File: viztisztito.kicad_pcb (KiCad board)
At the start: 2 copper layers, 110 x 102 mm, 77 parts, among them P1 BOARD_CONN, Q1 BC850, U1 VTX-214-010-205, U2 LTV-847, U3 ACS722, U4 MCP3004, U5 TC77

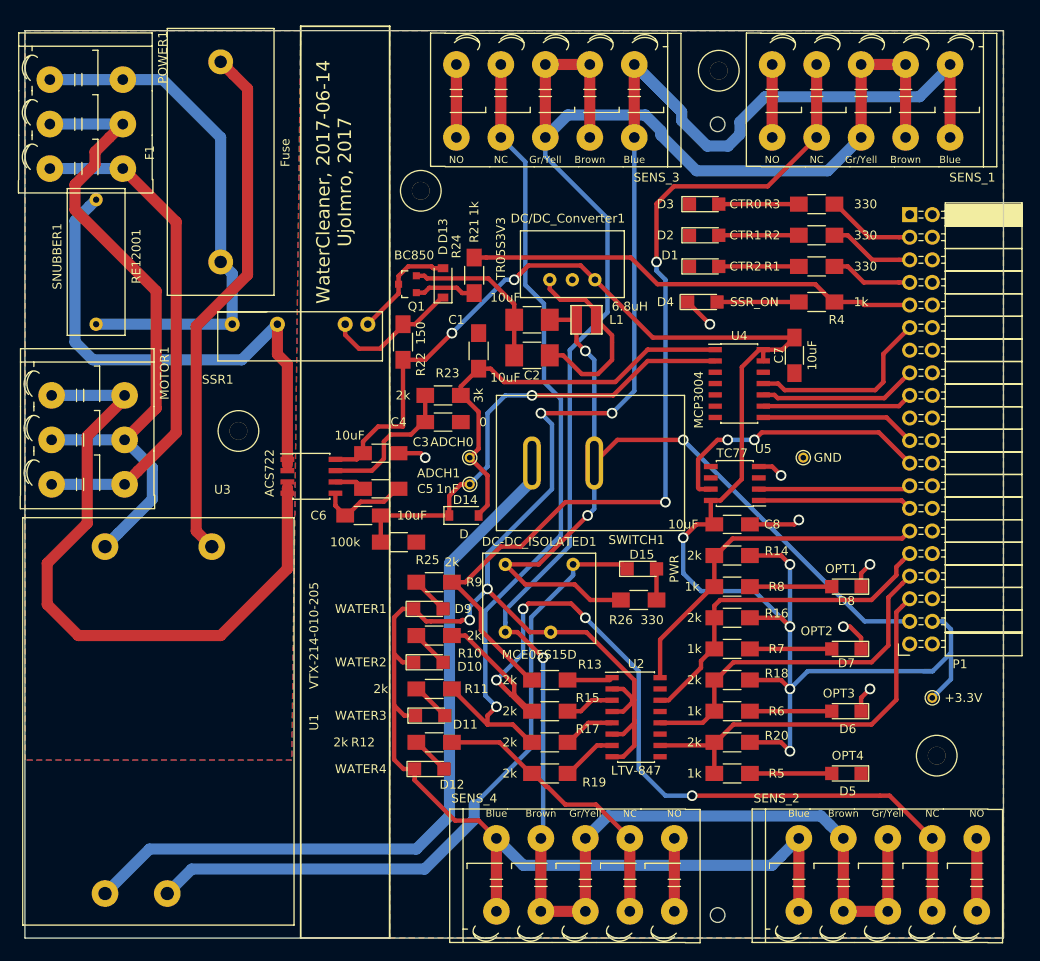
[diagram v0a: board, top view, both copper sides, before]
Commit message: final commit before manufacturing
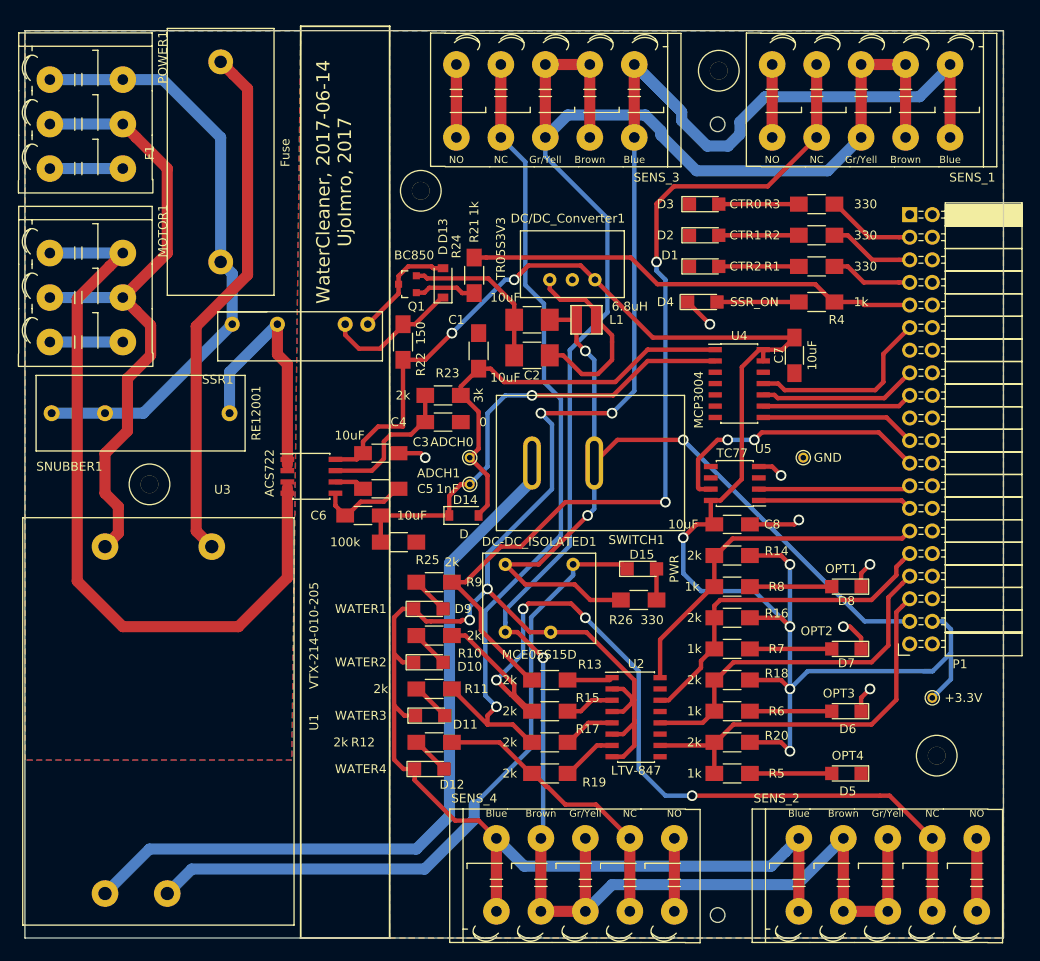
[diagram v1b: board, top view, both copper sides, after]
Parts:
- moved SNUBBER1 25.1 mm to (48.8, 70.2), turned to 180 degrees
- moved MOTOR1 16.0 mm to (30.0, 45.5)
- moved REF** 11.7 mm to (38.0, 74.0)
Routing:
- net 230V_GND: track 56.8 -> 16.4 mm
- net Net-(SNUBBER1-Pad1): track 59.5 -> 29.5 mm
- net /MOTOR+: track 77.0 -> 86.3 mm
- net 230V_AC+: track 58.7 -> 67.9 mm
- net 230V_NEUTRAL: track 74.9 -> 72.7 mm
- net /water_level/ISOLATED_+15V: track 246.8 -> 248.1 mm
